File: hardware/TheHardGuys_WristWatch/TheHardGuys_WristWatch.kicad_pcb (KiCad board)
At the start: 2 copper layers, 82 x 52.5 mm, 8 parts, among them P1 MB102 Output

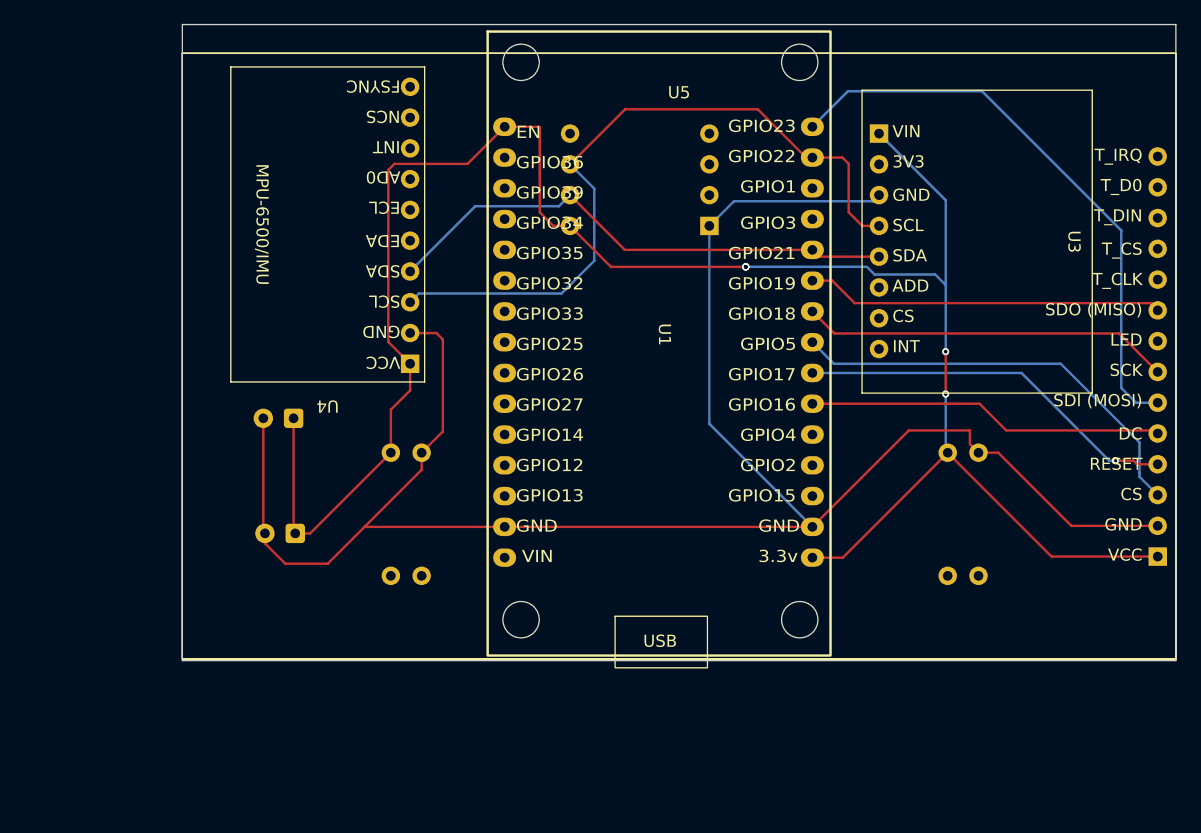
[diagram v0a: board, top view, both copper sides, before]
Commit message: Save Cause im scared
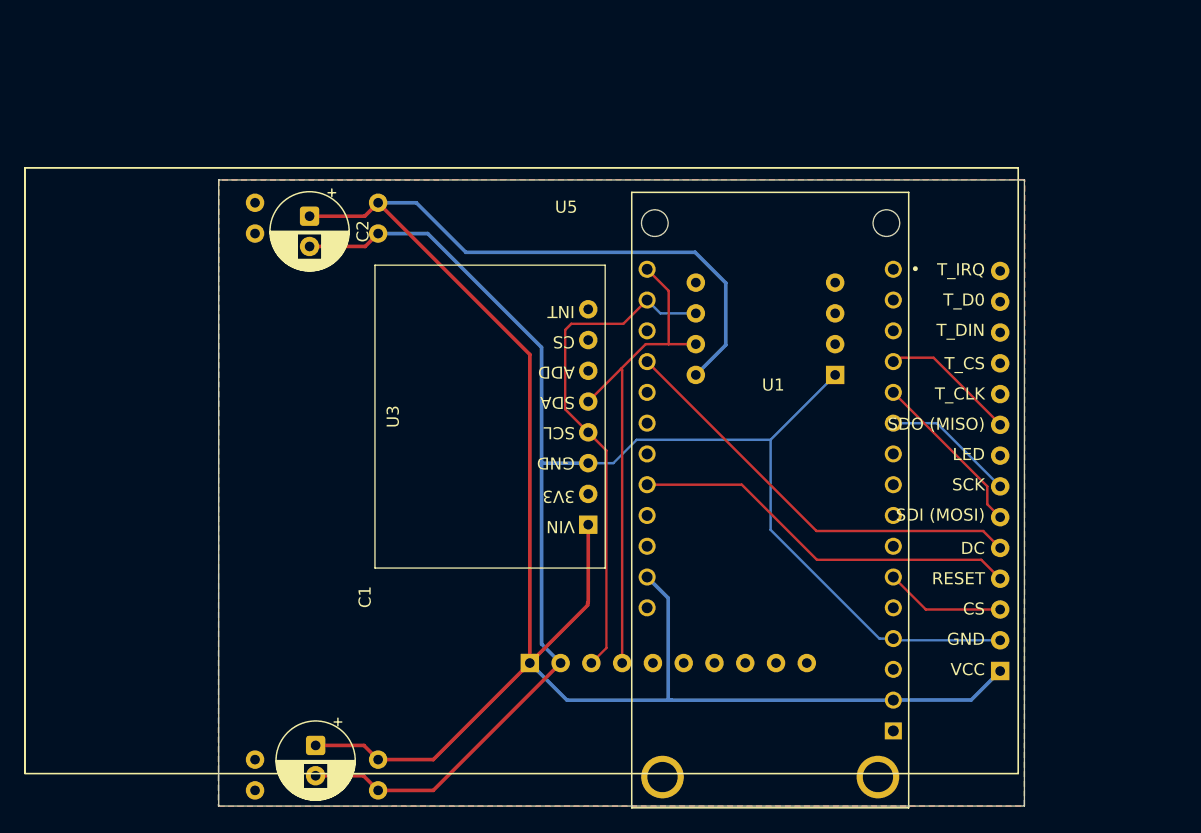
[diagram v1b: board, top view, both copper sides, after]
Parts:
- C1, C2: moved to F.Cu
- U1: footprint THG_Wristwatch:ESP32_30pin -> THG_Wristwatch:ESP32_Feather_V2
- U4: moved to B.Cu
- moved U4 51.4 mm to (124.2, 128.5), turned to -90 degrees
- moved U3 42.7 mm to (109.4, 101.4), turned to 90 degrees
- moved P1 33.2 mm to (92.5, 108.0), turned to -90 degrees
- moved C1 27.1 mm to (95.0, 128.5), turned to -90 degrees
- moved C2 26.2 mm to (94.5, 84.8), turned to -90 degrees
- moved U2 16.1 mm to (132.2, 94.0)
- moved U5 16.1 mm to (112.0, 105.8)
- moved U1 15.8 mm to (132.8, 108.0)
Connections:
- U1 pad 11: unconnected-(U1-GPIO35-Pad11) -> /SPI_SCK
- U1 pad 12: unconnected-(U1-GPIO34-Pad12) -> /SPI_MOSI
- U1 pad 13: unconnected-(U1-GPIO39-Pad13) -> /SPI_MISO
- U1 pad 15: +3.3V -> unconnected-(U1-TX/IO8-Pad15)
- U1 pad 16: +3.3V -> unconnected-(U1-D37/IO37-Pad16)
- U1 pad 17: GND -> /SDA
- U1 pad 18: unconnected-(U1-GPIO15-Pad18) -> /SCL
- U1 pad 2: GND -> +3.3V
- U1 pad 20: unconnected-(U1-GPIO4-Pad20) -> /SPI_DC
- U1 pad 21: /SPI_DC -> unconnected-(U1-D15/IO15-Pad21)
- U1 pad 22: /SPI_RST -> unconnected-(U1-D33/IO33-Pad22)
- U1 pad 23: /SPI_CS_LCD -> unconnected-(U1-D27/IO27-Pad23)
- U1 pad 24: /SPI_SCK -> /SPI_RST
- U1 pad 25: /SPI_MISO -> unconnected-(U1-LED/IO13-Pad25)
- U1 pad 26: /SDA -> unconnected-(U1-VBUS-Pad26)
- U1 pad 27: unconnected-(U1-GPIO3-Pad27) -> +3.3V
- U1 pad 4: unconnected-(U1-GPIO12-Pad4) -> GND
- U1 pad 6: unconnected-(U1-GPIO27-Pad6) -> /SPI_CS_LCD
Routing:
- net /SPI_MOSI: track 48.0 -> 14.0 mm
- net /SPI_CS_LCD: track 35.6 -> 9.93 mm
- net GND: track 157.7 -> 132.7 mm
- net /SPI_SCK: track 30.6 -> 11.0 mm
- net /SPI_MISO: track 29.5 -> 11.3 mm
- net /SCL: track 59.1 -> 41.7 mm
- net +3.3V: track 166.3 -> 176.5 mm, vias 5 -> 0
- net /SPI_DC: track 29.5 -> 35.5 mm
- net /SDA: track 43.4 -> 42.1 mm
- net /SPI_RST: track 31.6 -> 32.4 mm, vias 1 -> 0
- added copper zone on B.Cu, net GND
- added copper zone on F.Cu, net GND
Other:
- board size 82 x 52.5 mm -> 66.5 x 51.7 mm
